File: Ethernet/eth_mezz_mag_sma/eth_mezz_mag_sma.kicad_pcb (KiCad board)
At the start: 2 copper layers, 50 x 41 mm, 14 parts, among them J1 Conn_01x09_Male, J2 TX-, J3 RX+, J4 RX-, J5 TX+, J6 Conn_Coaxial

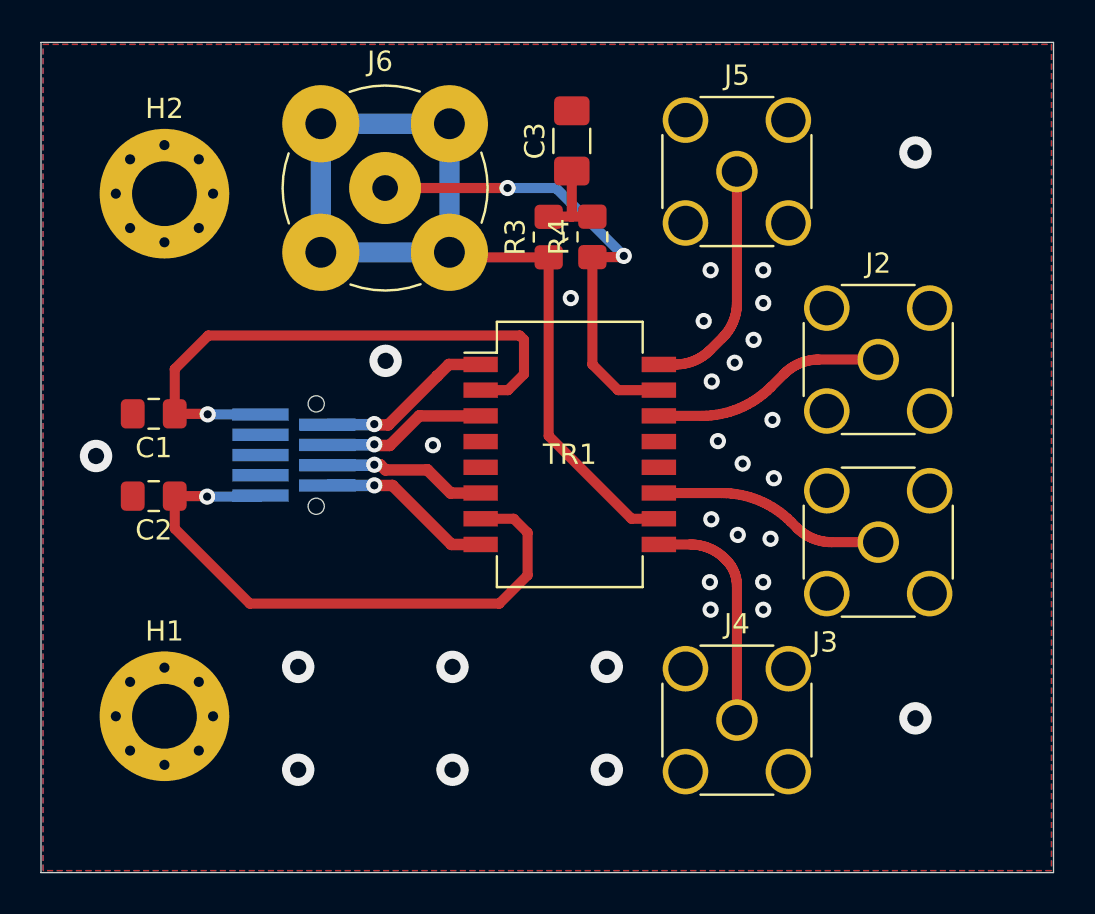
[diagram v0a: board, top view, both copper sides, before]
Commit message: FirstRoundPanelsDone
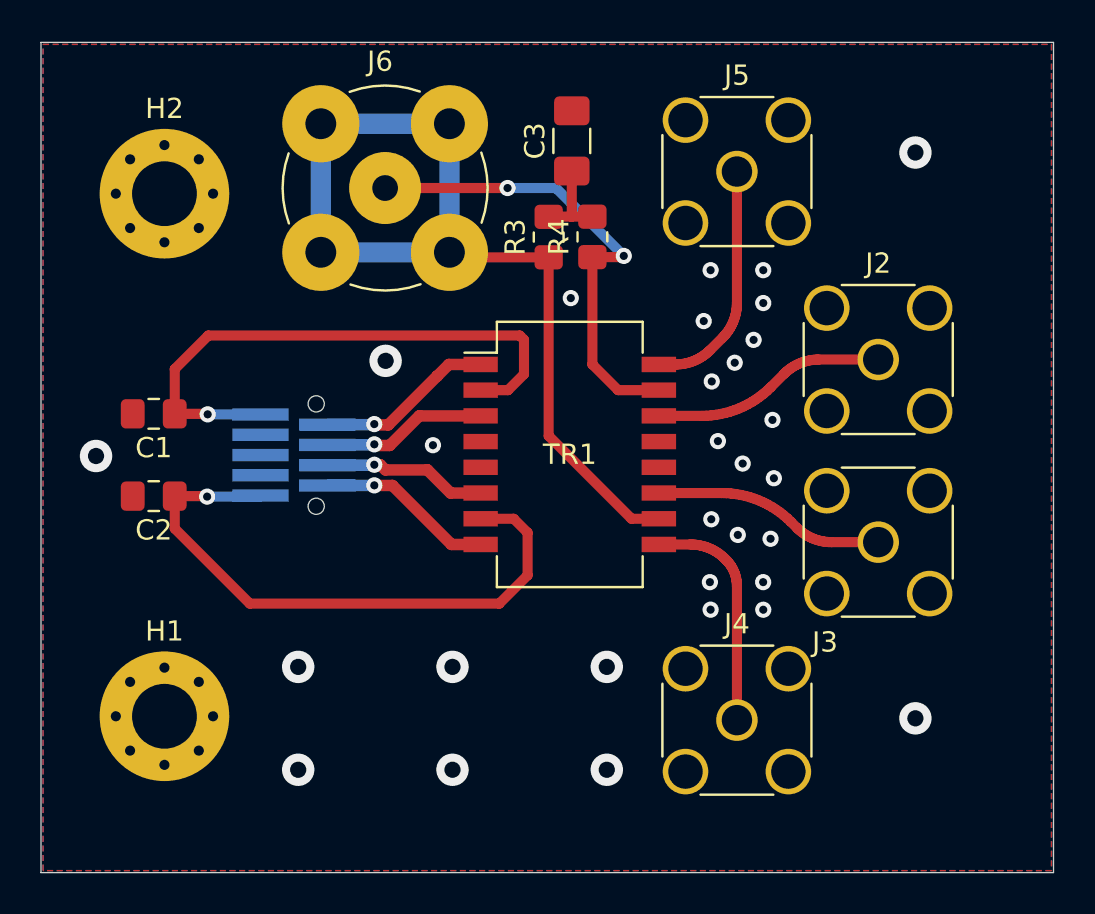
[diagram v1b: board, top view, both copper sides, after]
